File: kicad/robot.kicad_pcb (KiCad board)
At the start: 2 copper layers, 71.7 x 62.3 mm, 64 parts, among them J1 Adafruit Coil Jumper, J2 Adafruit Coil Jumper, J3 Adafruit Coil Jumper, J4 Adafruit Coil Jumper, M5 Motor_DC, M6 Motor_DC, M7 Motor_DC, M8 Motor_DC, Q2 NMOS, U10 GY-521, U13 DRV8833PW, U6 DRV8833PW, U8 ESP32-DEVKITC, U9 MCP73831-2-OT

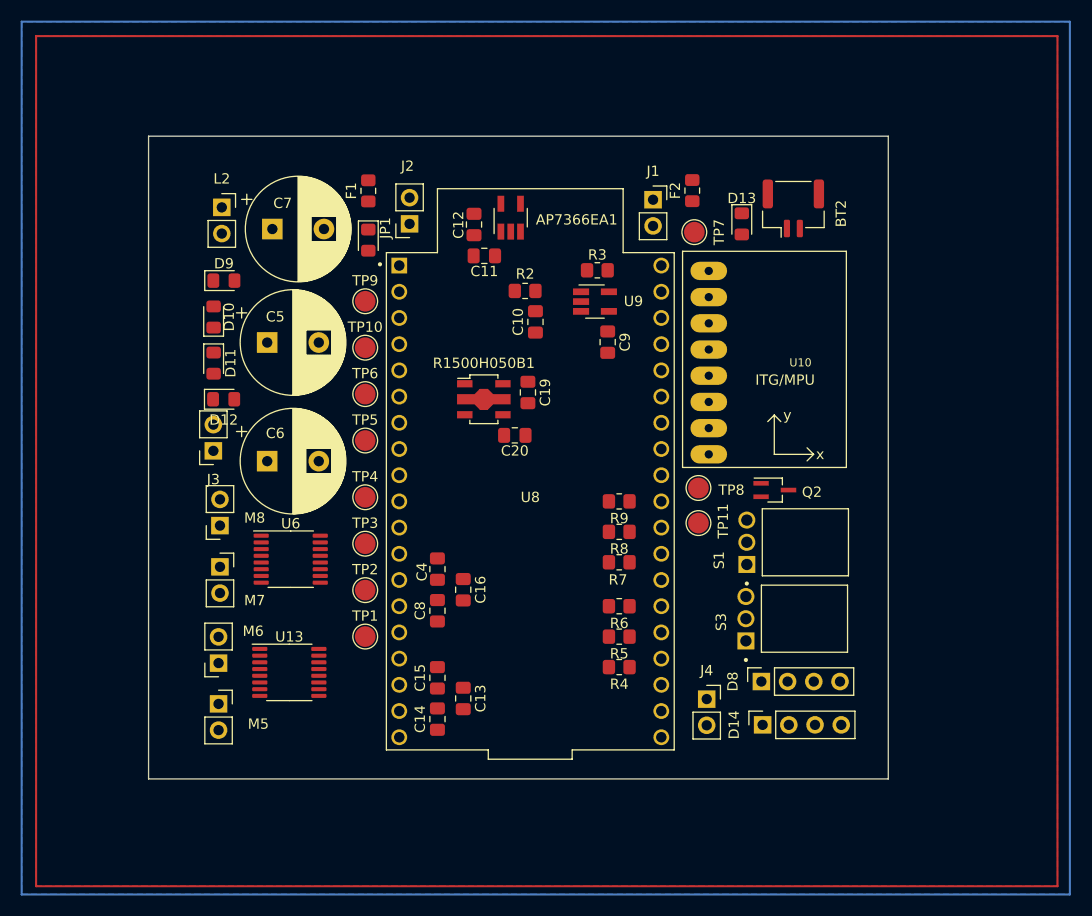
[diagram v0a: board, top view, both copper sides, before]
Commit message: First PCB Layout complete
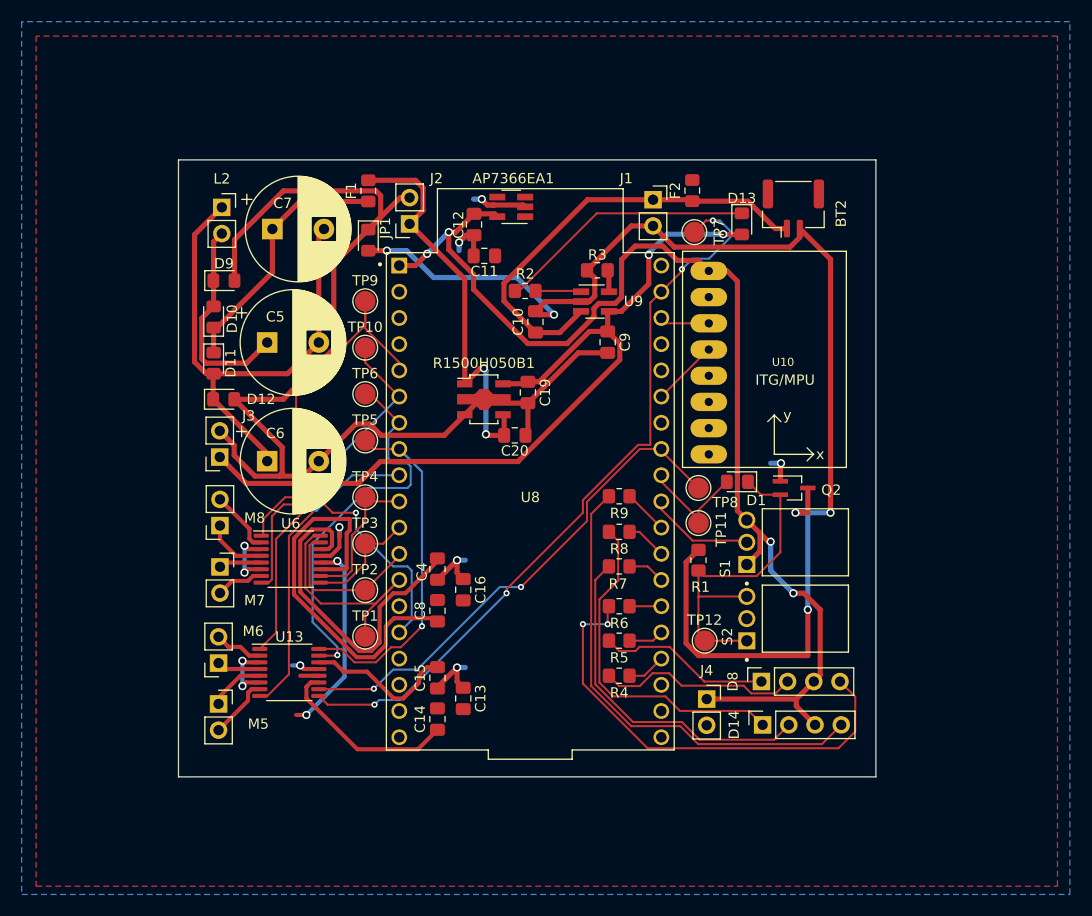
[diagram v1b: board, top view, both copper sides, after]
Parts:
- removed S3: TM1000Q, TM1000Q:SW_TM1000Q
- added D1: D, Diode_SMD:D_0805_2012Metric_Pad1.15x1.40mm_HandSolder, F.Cu at (210.6, 87.0)
- added R1: 2k, Resistor_SMD:R_0805_2012Metric_Pad1.20x1.40mm_HandSolder, F.Cu at (206.8, 94.6)
- added S2: TM1000Q, TM1000Q:SW_TM1000Q, F.Cu at (211.5, 100.3)
- added TP12: TestPoint, TestPoint:TestPoint_Pad_D2.0mm, F.Cu at (207.4, 102.4)
- moved Q2 1.88 mm to (216.1, 87.6)
- moved AP7366EA1 1.05 mm to (188.7, 60.4), turned to 180 degrees
- moved J3 0.86 mm to (160.4, 84.6)
- moved R4 0.84 mm to (199.1, 105.8)
- moved R9 0.50 mm to (199.1, 88.4)
- moved R7 0.40 mm to (199.1, 95.2)
- moved R5 0.39 mm to (199.1, 102.4)
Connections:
- Q2 pad 1: Net-(BT2--) -> /Temporary/Controller/GND
- Q2 pad 2: /Temporary/Controller/MOSTRIG -> Net-(D1-K)
- Q2 pad 3: Net-(Q2-S) -> Net-(BT2--)
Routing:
- net Net-(BT2--): track 0.00 -> 127.6 mm, vias 0 -> 5
- net /Temporary/Controller/3V3: track 0.00 -> 114.9 mm, vias 0 -> 4
- net Net-(D12-A): track 0.00 -> 112.8 mm
- net Net-(D13-A): track 0.00 -> 80.0 mm, vias 0 -> 2
- net Net-(U13-BIN1): track 0.00 -> 73.1 mm, vias 0 -> 4
- net Net-(D11-A): track 0.00 -> 51.7 mm
- net Net-(U13-BIN2): track 0.00 -> 49.2 mm, vias 0 -> 2
- net Net-(D14-RK): track 0.00 -> 46.4 mm
- net Net-(D8-RK): track 0.00 -> 45.1 mm, vias 0 -> 2
- net /Temporary/Controller/GND: track 0.00 -> 44.4 mm, vias 0 -> 11
- net Net-(BT2-+): track 0.00 -> 43.2 mm
- net Net-(U13-nFAULT): track 0.00 -> 41.1 mm, vias 0 -> 1
- net Net-(U6-nFAULT): track 0.00 -> 40.7 mm, vias 0 -> 2
- net Net-(J2-Pin_1): track 0.00 -> 40.2 mm, vias 0 -> 2
- net Net-(U6-VCP): track 0.00 -> 38.3 mm
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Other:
- board size 71.7 x 62.3 mm -> 67.6 x 59.8 mm
